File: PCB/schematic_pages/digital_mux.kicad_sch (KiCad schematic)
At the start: 9 parts

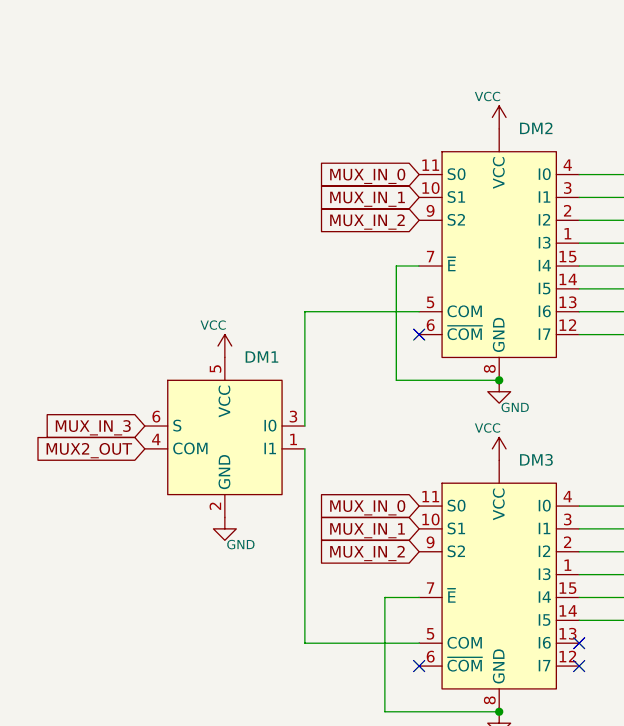
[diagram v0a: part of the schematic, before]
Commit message: repo rearrange
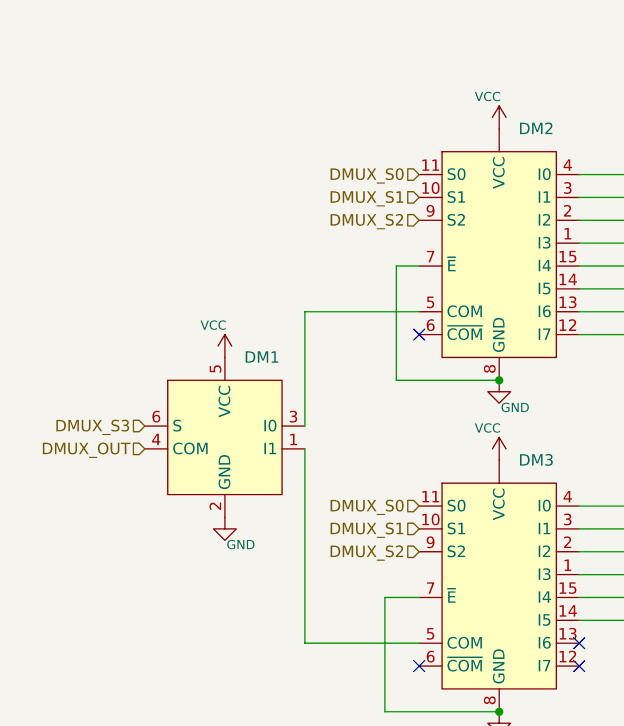
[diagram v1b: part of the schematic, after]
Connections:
- net MUX2_OUT renamed DMUX_OUT
- net MUX_IN_0 renamed DMUX_S0
- net MUX_IN_1 renamed DMUX_S1
- net MUX_IN_2 renamed DMUX_S2
- net MUX_IN_3 renamed DMUX_S3

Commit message: new schematics
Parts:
- DM1: footprint (none) -> Footprints:74LVC1G157 SOT-363 2_1 MUX
- DM2, DM3: footprint (none) -> Footprints:74AC151SC SOIC-16 8_1 MUX
- EN1, EN2, EN3, EN4, EN5, EN6: footprint (none) -> Footprints:Rotary Encoder EC11E
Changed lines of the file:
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@@
 			)
 		)
-		(property "Footprint" ""
+		(property "Footprint" "Footprints:Rotary Encoder EC11E"
 			(at 199.39 62.23 0)
 			(effects
@@
 			)
 		)
-		(property "Footprint" ""
+		(property "Footprint" "Footprints:Rotary Encoder EC11E"
 			(at 138.43 62.23 0)
 			(effects
@@
 			)
 		)
-		(property "Footprint" ""
+		(property "Footprint" "Footprints:74AC151SC SOIC-16 8_1 MUX"
 			(at 93.98 83.82 0)
 			(effects
@@
 			)
 		)
-		(property "Footprint" ""
+		(property "Footprint" "Footprints:Rotary Encoder EC11E"
 			(at 158.75 62.23 0)
 			(effects
@@
 			)
 		)
-		(property "Footprint" ""
+		(property "Footprint" "Footprints:Rotary Encoder EC11E"
 			(at 179.07 62.23 0)
 			(effects
@@
 			)
 		)
-		(property "Footprint" ""
+		(property "Footprint" "Footprints:74LVC1G157 SOT-363 2_1 MUX"
 			(at 63.5 106.68 0)
 			(effects
@@
 			)
 		)
-		(property "Footprint" ""
+		(property "Footprint" "Footprints:Rotary Encoder EC11E"
 			(at 118.11 62.23 0)
 			(effects
@@
 			)
 		)
-		(property "Footprint" ""
+		(property "Footprint" "Footprints:Rotary Encoder EC11E"
 			(at 219.71 62.23 0)
 			(effects
@@
 			)
 		)
-		(property "Footprint" ""
+		(property "Footprint" "Footprints:74AC151SC SOIC-16 8_1 MUX"
 			(at 93.98 120.65 0)
 			(effects
